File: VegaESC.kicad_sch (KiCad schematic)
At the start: 59 parts, among them J201 A, J202 B, J203 C, Q201 NTMFS5C430NLT1G, Q202 NTMFS5C430NLT1G, Q203 NTMFS5C430NLT1G, Q204 NTMFS5C430NLT1G, Q205 NTMFS5C430NLT1G, Q206 NTMFS5C430NLT1G, U202 FD6288Q, U203 AT32F421G8U7

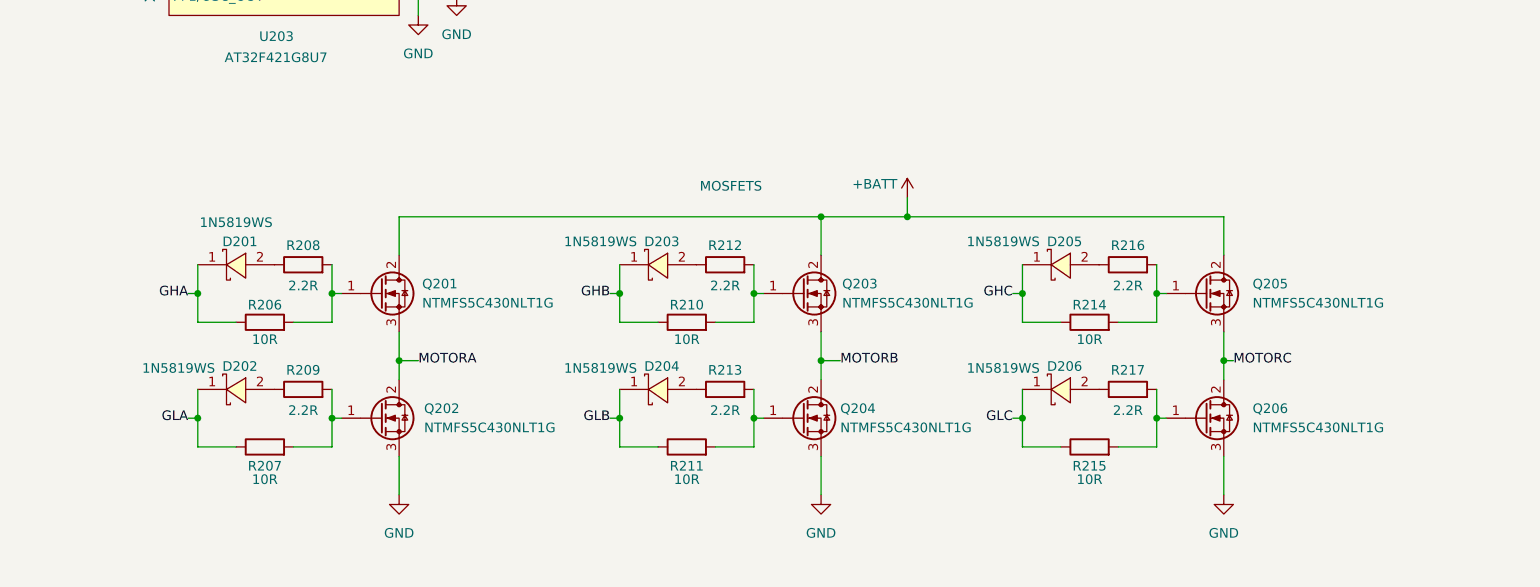
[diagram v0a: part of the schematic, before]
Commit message: Stage user updates for MOSFET pinouts and MCU footprints, and update design review
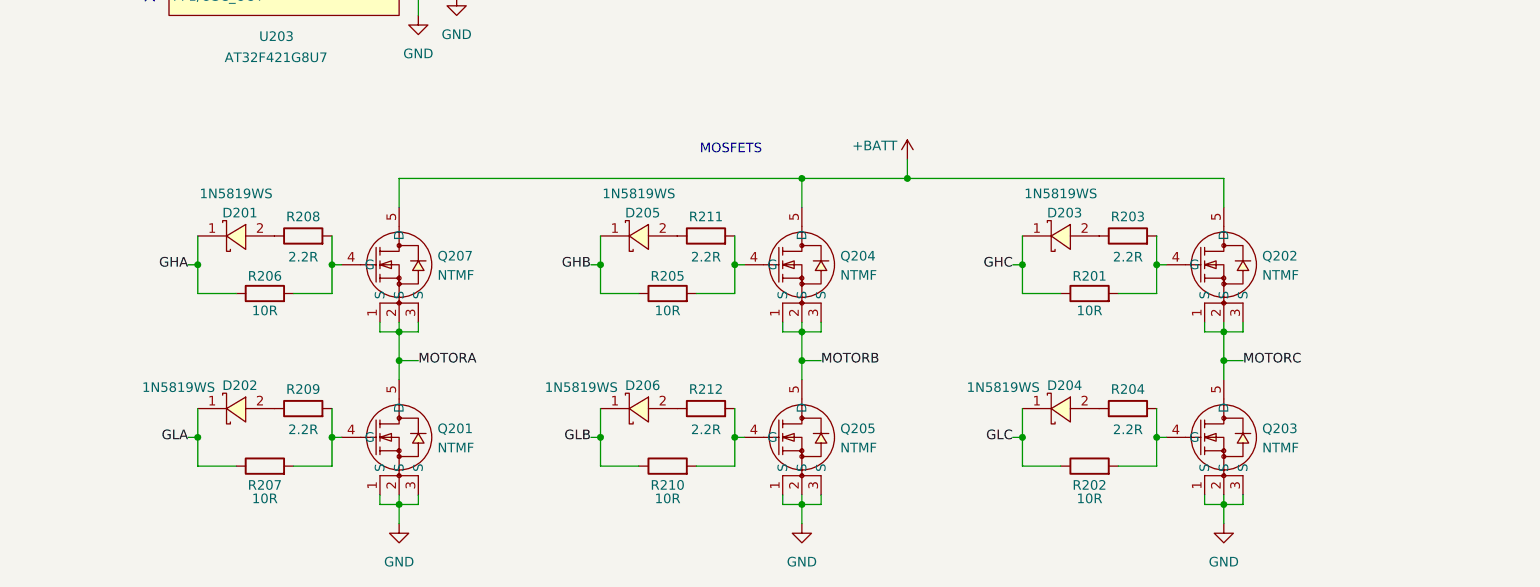
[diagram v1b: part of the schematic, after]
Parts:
- removed Q201, Q202, Q203, Q204, Q205, Q206: NTMFS5C430NLT1G, easyeda2kicad:DFN-5_L4.9-W5.9-P1.27-LS6.2-BL, symbol Transistor_FET:Q_NMOS_GDS
- removed R213, R216, R217: 2.2R, Resistor_SMD:R_0603_1608Metric, symbol Device:R
- removed R214, R215: 10R, Resistor_SMD:R_0603_1608Metric, symbol Device:R
- added Q201, Q202, Q203, Q204, Q205, Q207: NTMF, easyeda2kicad:DFN-5_L4.9-W5.9-P1.27-LS6.2-BL, symbol easyeda2kicad:NTMFS5C430NLT1G
- added R201, R202, R205: 10R, Resistor_SMD:R_0603_1608Metric, symbol Device:R
- added R203, R204: 2.2R, Resistor_SMD:R_0603_1608Metric, symbol Device:R
- R211: value 10R -> 2.2R; MPN 0603WAF100JT5E -> 0603WAF220JT5E; lcsc C22859 -> C25877
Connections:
- net +BATT: now also Q202.5 (D), Q204.5 (D), Q207.5 (D)
- net GHB: now also D205.1, R205.1; no longer D203.1, R210.1
- net GHC: now also D203.1, R201.1; no longer D205.1
- net GLB: now also D206.1, R210.1; no longer D204.1, R211.1
- net GLC: now also D204.1, R202.1; no longer D206.1
- net GND: now also Q201.1 (S), Q201.2 (S), Q201.3 (S), Q203.1 (S), Q203.2 (S), Q203.3 (S), Q205.1 (S), Q205.2 (S), Q205.3 (S)
- net MOTORA: now also Q201.5 (D), Q207.1 (S), Q207.2 (S), Q207.3 (S)
- net MOTORB: now also Q204.1 (S), Q204.2 (S), Q204.3 (S), Q205.5 (D)
- net MOTORC: now also Q202.1 (S), Q202.2 (S), Q202.3 (S), Q203.5 (D)
- net at D206.2: now also R212.1
- net at R207.2, R209.2: now also Q201.4 (G)
- net at D205.2: now also R211.1
- net at R210.2, R212.2: now also Q205.4 (G)
- net at D204.2: now also R204.1
- net at R211.2: now also Q204.4 (G), R205.2
- net at R206.2, R208.2: now also Q207.4 (G)
- net at D203.2: now also R203.1; no longer R212.1
- new net: Q203.4 (G), R202.2, R204.2
- new net: Q202.4 (G), R201.2, R203.2
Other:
- moved on the sheet: D201, D202, R206, R207, R208, R209
